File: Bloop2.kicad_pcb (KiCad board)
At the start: 2 copper layers, 15 parts, among them J1 Input, J2 Output, U1 TL072

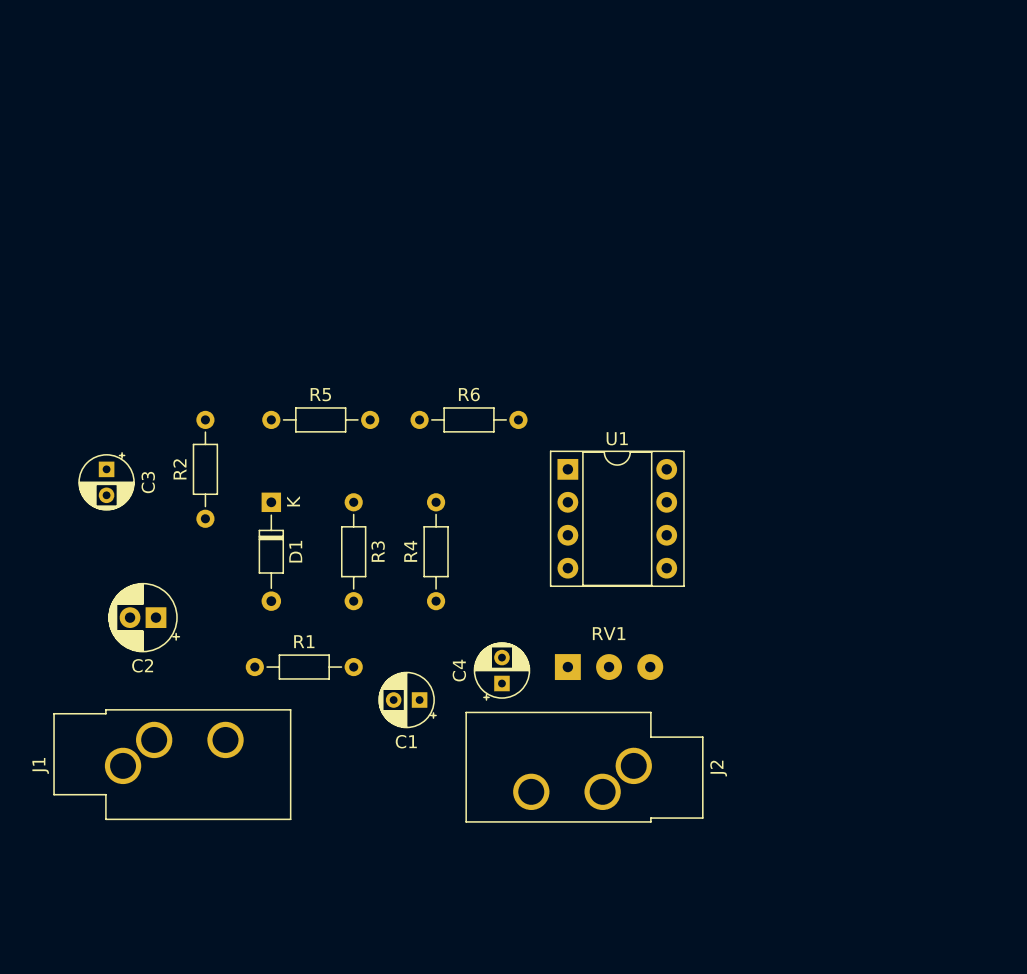
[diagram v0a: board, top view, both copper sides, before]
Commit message: Feature complete device with first layout.
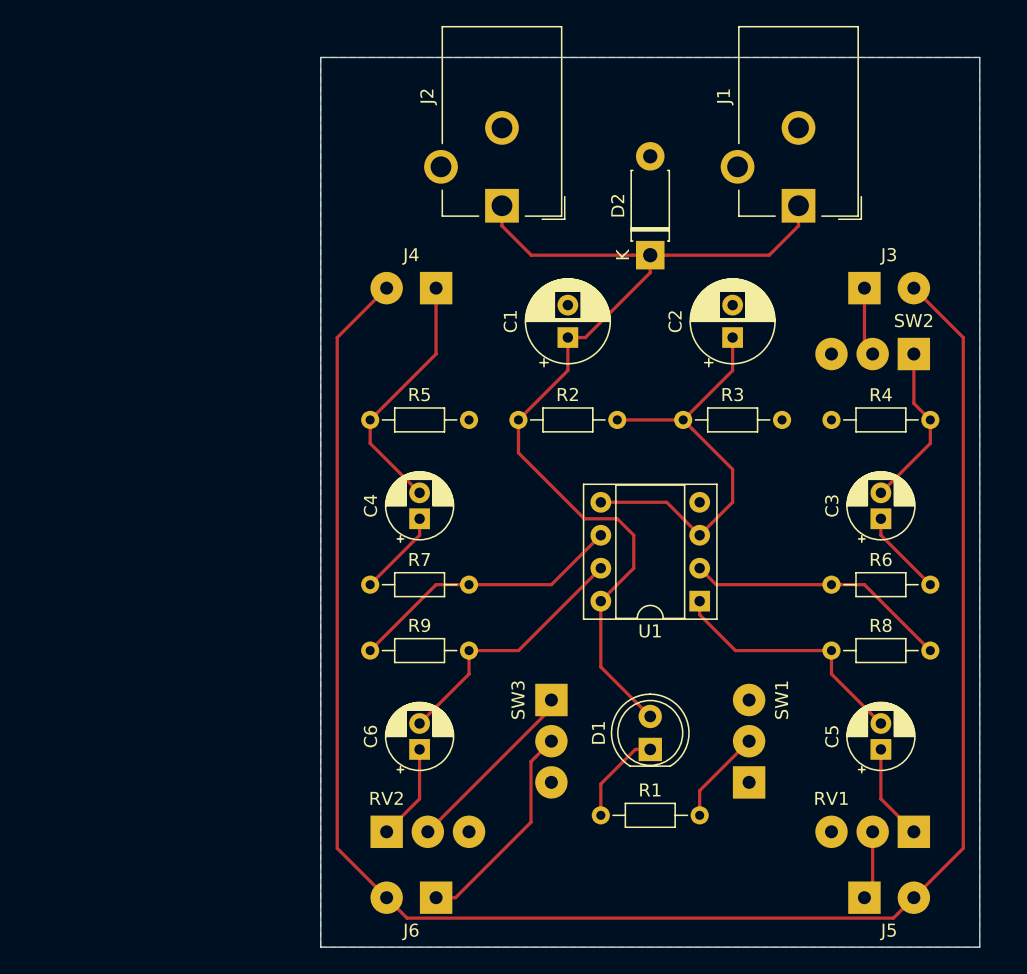
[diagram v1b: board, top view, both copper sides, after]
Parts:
- added C5: 1u, Capacitor_THT:CP_Radial_D5.0mm_P2.00mm, F.Cu at (171.4, 118.1)
- added C6: 1u, Capacitor_THT:CP_Radial_D5.0mm_P2.00mm, F.Cu at (135.9, 118.1)
- added D2: D, Diode_THT:D_DO-41_SOD81_P7.62mm_Horizontal, F.Cu at (153.7, 80.0)
- added J3: Input, Connector_Wire:SolderWirePad_1x02_P3.81mm_Drill1mm, F.Cu at (170.2, 82.5)
- added J4: Return, Connector_Wire:SolderWirePad_1x02_P3.81mm_Drill1mm, F.Cu at (137.2, 82.5)
- added J5: Send, Connector_Wire:SolderWirePad_1x02_P3.81mm_Drill1mm, F.Cu at (170.2, 129.5)
- added J6: Output, Connector_Wire:SolderWirePad_1x02_P3.81mm_Drill1mm, F.Cu at (137.2, 129.5)
- added R7: 10k, Resistor_THT:R_Axial_DIN0204_L3.6mm_D1.6mm_P7.62mm_Horizontal, F.Cu at (132.1, 105.4)
- added R8: 47k, Resistor_THT:R_Axial_DIN0204_L3.6mm_D1.6mm_P7.62mm_Horizontal, F.Cu at (175.3, 110.5)
- added R9: 47k, Resistor_THT:R_Axial_DIN0204_L3.6mm_D1.6mm_P7.62mm_Horizontal, F.Cu at (132.1, 110.5)
- added RV2: 10k, Connector_Wire:SolderWirePad_1x03_P3.175mm_Drill1mm, F.Cu at (133.3, 124.5)
- added SW1: 3PDT-A, Connector_Wire:SolderWirePad_1x03_P3.175mm_Drill1mm, F.Cu at (161.3, 120.7)
- added SW2: 3PDT-B, Connector_Wire:SolderWirePad_1x03_P3.175mm_Drill1mm, F.Cu at (174.0, 87.6)
- added SW3: 3PDT-C, Connector_Wire:SolderWirePad_1x03_P3.175mm_Drill1mm, F.Cu at (146.1, 114.3)
- C1: value 1u -> 47u; footprint Capacitor_THT:CP_Radial_D4.0mm_P2.00mm -> Capacitor_THT:CP_Radial_D6.3mm_P2.50mm
- C2: value 100u -> 47u; footprint Capacitor_THT:CP_Radial_D5.0mm_P2.00mm -> Capacitor_THT:CP_Radial_D6.3mm_P2.50mm
- C3: value 47u -> 1u; footprint Capacitor_THT:CP_Radial_D4.0mm_P2.00mm -> Capacitor_THT:CP_Radial_D5.0mm_P2.00mm
- C4: footprint Capacitor_THT:CP_Radial_D4.0mm_P2.00mm -> Capacitor_THT:CP_Radial_D5.0mm_P2.00mm
- D1: value D -> LED; footprint Diode_THT:D_DO-34_SOD68_P7.62mm_Horizontal -> LED_THT:LED_D5.0mm
- J1: value Input -> Power In; footprint Connector_Audio:Jack_3.5mm_CUI_SJ1-3533NG_Horizontal_CircularHoles -> Connector_BarrelJack:BarrelJack_CUI_PJ-102AH_Horizontal
- J2: value Output -> Power Out; footprint Connector_Audio:Jack_3.5mm_CUI_SJ1-3533NG_Horizontal_CircularHoles -> Connector_BarrelJack:BarrelJack_CUI_PJ-102AH_Horizontal
- R1: value 100k -> 2k7
- R4, R5: value 10k -> 100k
- R6: value 22k -> 10k
- RV1: footprint Connector_Wire:SolderWirePad_1x03_P3.175mm_Drill0.8mm -> Connector_Wire:SolderWirePad_1x03_P3.175mm_Drill1mm
- moved J1 67.6 mm to (165.1, 76.2), turned to 180 degrees
- moved C3 59.8 mm to (171.4, 100.3), turned to 90 degrees
- moved C2 49.4 mm to (160.0, 86.4), turned to 90 degrees
- moved J2 44.4 mm to (142.2, 76.2), turned to 180 degrees
- moved R6 41.4 mm to (175.3, 105.4), turned to 180 degrees
- moved R4 40.6 mm to (175.3, 92.7), turned to 180 degrees
- moved D1 34.9 mm to (153.7, 118.1), turned to 90 degrees
- moved C1 30.2 mm to (147.3, 86.4), turned to 90 degrees
- moved RV1 29.5 mm to (174.0, 124.5), turned to 180 degrees
- moved R1 29.0 mm to (149.9, 123.2)
- moved R3 26.2 mm to (156.2, 92.7), turned to 0 degrees
- moved R2 25.3 mm to (143.5, 92.7), turned to 0 degrees
- moved U1 14.4 mm to (157.5, 106.7), turned to 180 degrees
- moved C4 14.2 mm to (135.9, 100.3)
- moved R5 7.62 mm to (132.1, 92.7)
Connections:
- C1 pad 1: Net-(C1-Pad1) -> +9V
- C1 pad 2: Net-(C1-Pad2) -> GND
- C2 pad 1: +9V -> VREF
- C3 pad 2: GND -> Net-(C3-Pad2)
- D1 pad 1: +9V -> Net-(D1-Pad1)
- D1 pad 2: GND -> +9V
- R1 pad 1: Net-(C1-Pad2) -> Net-(D1-Pad1)
- R1 pad 2: GND -> Net-(R1-Pad2)
- R2 pad 2: Net-(C3-Pad1) -> VREF
- R3 pad 1: Net-(C3-Pad1) -> VREF
- R4 pad 1: Net-(C1-Pad1) -> Net-(C3-Pad2)
- R4 pad 2: Net-(C3-Pad1) -> GND
- R5 pad 1: Net-(C3-Pad1) -> Net-(C4-Pad2)
- R5 pad 2: Net-(R5-Pad2) -> GND
- R6 pad 1: Net-(R5-Pad2) -> Net-(C3-Pad1)
- R6 pad 2: Net-(C4-Pad2) -> Net-(R6-Pad2)
- RV1 pad 1: Net-(C4-Pad1) -> Net-(C5-Pad1)
- RV1 pad 2: Net-(J2-PadT) -> Net-(J5-Pad1)
- U1 pad 1: Net-(C4-Pad2) -> Net-(C5-Pad2)
- U1 pad 2: Net-(R5-Pad2) -> Net-(R6-Pad2)
- U1 pad 3: Net-(C1-Pad1) -> VREF
- U1 pad 5: (no net) -> VREF
- U1 pad 6: (no net) -> Net-(R7-Pad2)
- U1 pad 7: (no net) -> Net-(C6-Pad2)
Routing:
- net GNDPWR: track 0.00 -> 142.2 mm
- net +9V: track 0.00 -> 76.2 mm
- net VREF: track 0.00 -> 33.2 mm
- net Net-(R7-Pad2): track 0.00 -> 21.5 mm
- net Net-(R6-Pad2): track 0.00 -> 20.4 mm
- net Net-(C6-Pad2): track 0.00 -> 20.0 mm
- net Net-(C5-Pad2): track 0.00 -> 19.6 mm
- net Net-(C4-Pad2): track 0.00 -> 19.5 mm
- net Net-(J6-Pad1): track 0.00 -> 16.6 mm
- net Net-(RV2-Pad2): track 0.00 -> 14.1 mm
- net Net-(C3-Pad2): track 0.00 -> 12.8 mm
- net Net-(R1-Pad2): track 0.00 -> 7.93 mm
- net Net-(C5-Pad1): track 0.00 -> 7.40 mm
- net Net-(C6-Pad1): track 0.00 -> 7.40 mm
- net Net-(D1-Pad1): track 0.00 -> 7.33 mm
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- added copper zone on B.Cu, net GND
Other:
- board outline added: 50.8 x 68.6 mm
- rule pad_to_mask_clearance: 0.051 -> 0

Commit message: Improved, compacted layout.
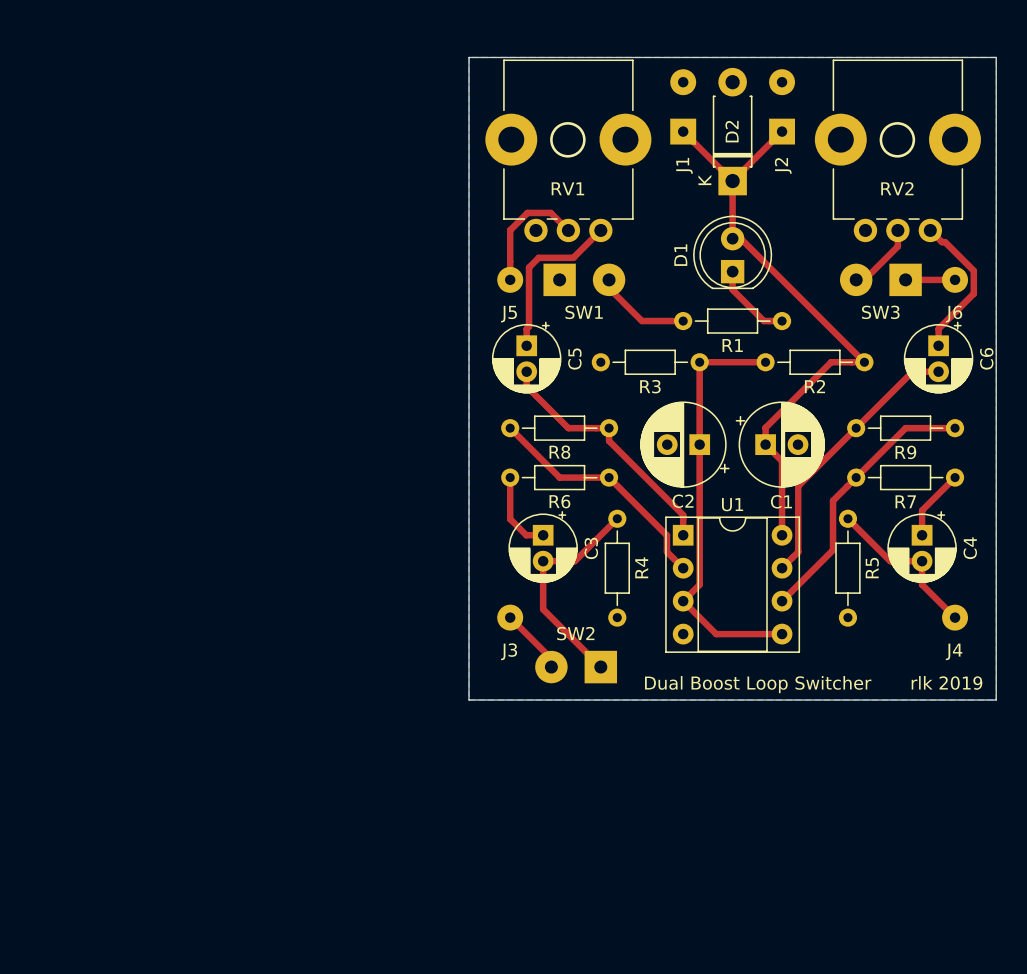
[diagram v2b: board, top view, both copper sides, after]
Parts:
- D2: value D -> 40V
- J1, J2: footprint Connector_BarrelJack:BarrelJack_CUI_PJ-102AH_Horizontal -> Connector_Wire:SolderWirePad_1x02_P3.81mm_Drill0.8mm
- J3, J4, J5, J6: footprint Connector_Wire:SolderWirePad_1x02_P3.81mm_Drill1mm -> Connector_Wire:SolderWirePad_1x01_Drill0.8mm
- R8, R9: value 47k -> 100k
- RV1, RV2: footprint Connector_Wire:SolderWirePad_1x03_P3.175mm_Drill1mm -> Potentiometer_THT:Potentiometer_Bourns_PTV09A-1_Single_Vertical
- SW1: value 3PDT-A -> 3PDTA; footprint Connector_Wire:SolderWirePad_1x03_P3.175mm_Drill1mm -> Connector_Wire:SolderWirePad_1x02_P3.81mm_Drill1mm
- SW2: value 3PDT-B -> 3PDTB; footprint Connector_Wire:SolderWirePad_1x03_P3.175mm_Drill1mm -> Connector_Wire:SolderWirePad_1x02_P3.81mm_Drill1mm
- SW3: value 3PDT-C -> 3PDTC; footprint Connector_Wire:SolderWirePad_1x03_P3.175mm_Drill1mm -> Connector_Wire:SolderWirePad_1x02_P3.81mm_Drill1mm
- moved RV2 62.5 mm to (175.3, 78.1), turned to 90 degrees
- moved J6 62.2 mm to (177.2, 81.9), turned to 0 degrees
- moved J5 54.9 mm to (142.9, 81.9)
- moved RV1 52.3 mm to (149.9, 78.1), turned to 90 degrees
- moved C6 50.7 mm to (175.9, 87.0), turned to 270 degrees
- moved R9 48.2 mm to (177.2, 93.3), turned to 180 degrees
- moved J4 47.4 mm to (177.2, 108.0), turned to 0 degrees
- moved R7 45.8 mm to (177.2, 97.2), turned to 180 degrees
- moved SW3 42.4 mm to (173.4, 81.9), turned to 180 degrees
- moved SW1 41.4 mm to (146.7, 81.9), turned to 0 degrees
- moved C5 41.4 mm to (144.1, 87.0), turned to 270 degrees
- moved R1 40.6 mm to (163.8, 85.1), turned to 180 degrees
- moved C4 38.8 mm to (174.6, 101.6), turned to 270 degrees
- moved R5 37.6 mm to (168.9, 100.3), turned to 270 degrees
- moved D1 37.4 mm to (160.0, 81.3)
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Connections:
- SW3 pad 1: Net-(RV2-Pad2) -> Net-(J6-Pad1)
- SW3 pad 2: Net-(J6-Pad1) -> Net-(RV2-Pad2)
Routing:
- net GNDPWR: track 142.2 -> 0.00 mm
- net +9V: track 76.2 -> 47.8 mm
- net Net-(J6-Pad1): track 16.6 -> 3.81 mm
- net Net-(RV2-Pad2): track 14.1 -> 4.88 mm
- net Net-(C4-Pad2): track 19.5 -> 12.5 mm
- net Net-(C5-Pad1): track 7.40 -> 12.8 mm
- net Net-(C3-Pad2): track 12.8 -> 17.1 mm
- net Net-(C6-Pad1): track 7.40 -> 11.5 mm
- net Net-(J5-Pad1): track 5.34 -> 9.42 mm
- net Net-(R6-Pad2): track 20.4 -> 18.6 mm
- net Net-(C6-Pad2): track 20.0 -> 21.3 mm
- net Net-(C4-Pad1): track 6.66 -> 5.53 mm
- net Net-(D1-Pad1): track 7.33 -> 6.21 mm
- net VREF: track 33.2 -> 32.7 mm
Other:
- board size 50.8 x 68.6 mm -> 40.6 x 49.5 mm
- net class Default: trace_width 0.25 -> 0.5
- board text added: "Dual Boost Loop Switcher"
- board text added: "rlk 2019"

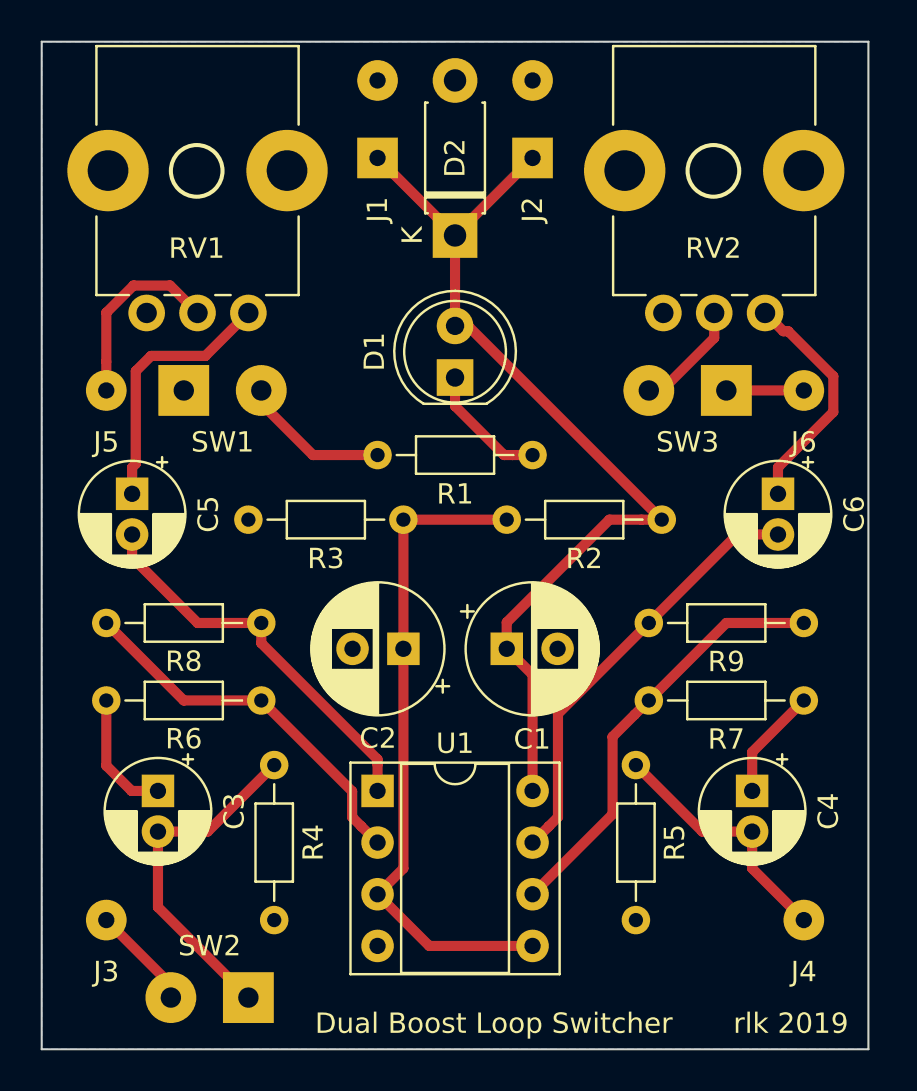
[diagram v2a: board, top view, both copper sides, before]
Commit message: Tuned layout.
The moment you send a PCB off for printing, you think of a ton of obvious ideas for improvement.
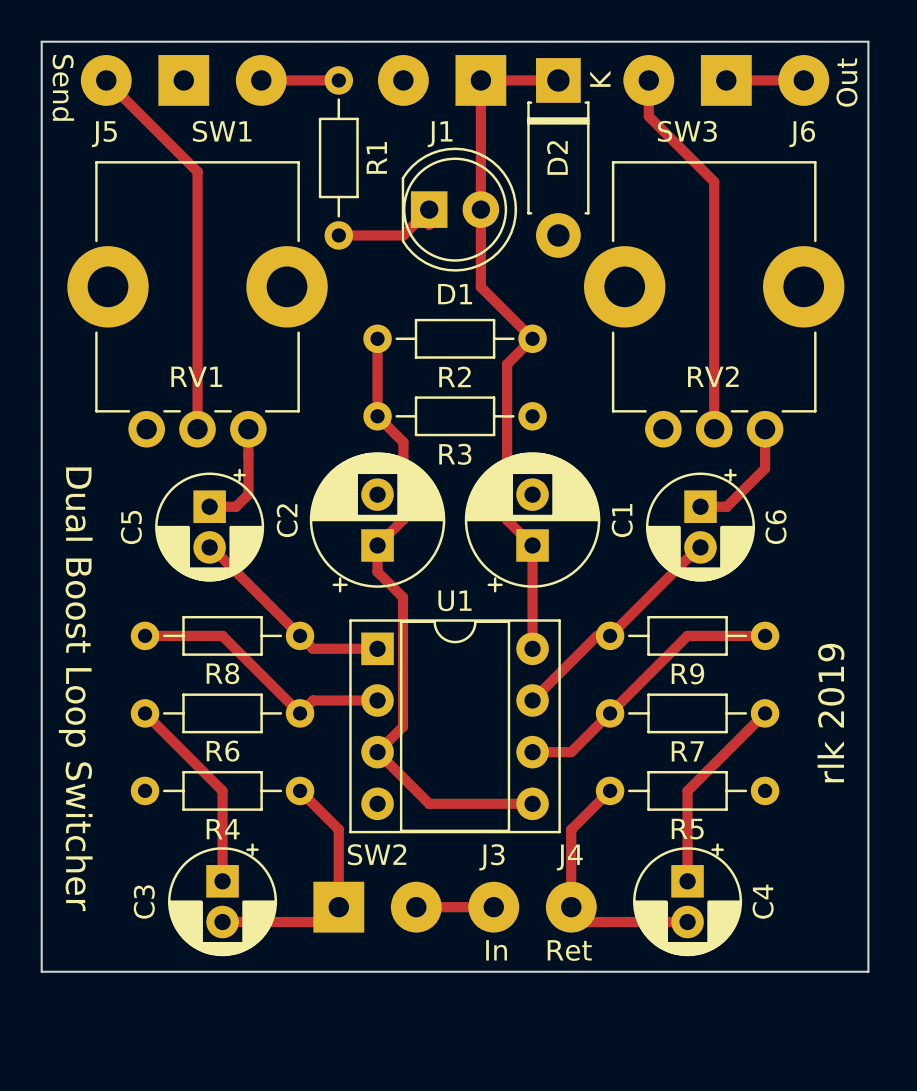
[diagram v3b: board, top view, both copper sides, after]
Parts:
- removed J2: Power Out, Connector_Wire:SolderWirePad_1x02_P3.81mm_Drill0.8mm
- J1: footprint Connector_Wire:SolderWirePad_1x02_P3.81mm_Drill0.8mm -> Connector_Wire:SolderWirePad_1x02_P3.81mm_Drill1mm
- J3, J4, J5, J6: footprint Connector_Wire:SolderWirePad_1x01_Drill0.8mm -> Connector_Wire:SolderWirePad_1x01_Drill1mm
- moved J3 19.1 mm to (161.9, 107.3)
- moved J5 15.2 mm to (142.9, 66.7)
- moved J6 15.2 mm to (177.2, 66.7)
- moved SW1 15.2 mm to (146.7, 66.7)
- moved SW3 15.2 mm to (173.4, 66.7)
- moved R1 14.4 mm to (154.3, 74.3), turned to 90 degrees
- moved J4 11.4 mm to (165.7, 107.3)
- moved R2 10.9 mm to (163.8, 79.4)
- moved D2 9.16 mm to (165.1, 66.7), turned to 270 degrees
- moved D1 8.35 mm to (158.8, 73.0), turned to 0 degrees
- moved U1 6.98 mm to (156.2, 94.6)
- moved J1 6.35 mm to (161.3, 66.7), turned to 180 degrees
- moved SW2 6.29 mm to (154.3, 107.3), turned to 0 degrees
- moved RV1 5.71 mm to (149.9, 83.8)
- moved RV2 5.71 mm to (175.3, 83.8)
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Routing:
- net +9V: track 47.8 -> 33.8 mm
- net Net-(RV2-Pad2): track 4.88 -> 18.5 mm
- net Net-(C6-Pad2): track 21.3 -> 11.4 mm
- net Net-(J5-Pad1): track 9.42 -> 19.0 mm
- net Net-(C5-Pad2): track 19.4 -> 10.3 mm
- net Net-(C5-Pad1): track 12.8 -> 5.36 mm
- net Net-(R7-Pad2): track 21.1 -> 13.8 mm
- net Net-(C6-Pad1): track 11.5 -> 5.89 mm
- net Net-(R6-Pad2): track 18.6 -> 13.3 mm
- net Net-(C3-Pad2): track 17.1 -> 12.5 mm
- net Net-(C4-Pad1): track 5.53 -> 9.83 mm
- net Net-(R1-Pad2): track 7.67 -> 3.81 mm
- net Net-(C3-Pad1): track 6.26 -> 9.83 mm
- net VREF: track 32.7 -> 31.1 mm
- net Net-(J3-Pad1): track 5.39 -> 3.81 mm
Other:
- board size 40.6 x 49.5 mm -> 40.6 x 45.7 mm
- board text added: "In"
- board text added: "Out"
- board text added: "Ret"
- board text added: "Send"
